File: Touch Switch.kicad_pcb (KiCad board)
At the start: 2 copper layers, 84.8 x 53.2 mm, 55 parts, among them J1 Conn_01x01_Pin, J2 Conn_02x04_Counter_Clockwise, J3 Conn_01x01_Pin, J4 Conn_01x01_Pin, J5 Conn_01x01_Pin, J6 Conn_01x01_Pin, J7 Conn_01x01_Pin, J8 Conn_01x01_Pin, K1 Relay_SPST-NO, K2 Relay_SPST-NO, K3 Relay_SPST-NO, K4 Relay_SPST-NO, Q1 MMBT3904, Q2 MMBT3904, Q3 MMBT3904, Q5 MMBT3904, T1 Transformer_1P_2S, U1 SCJT1117B-3.3-A

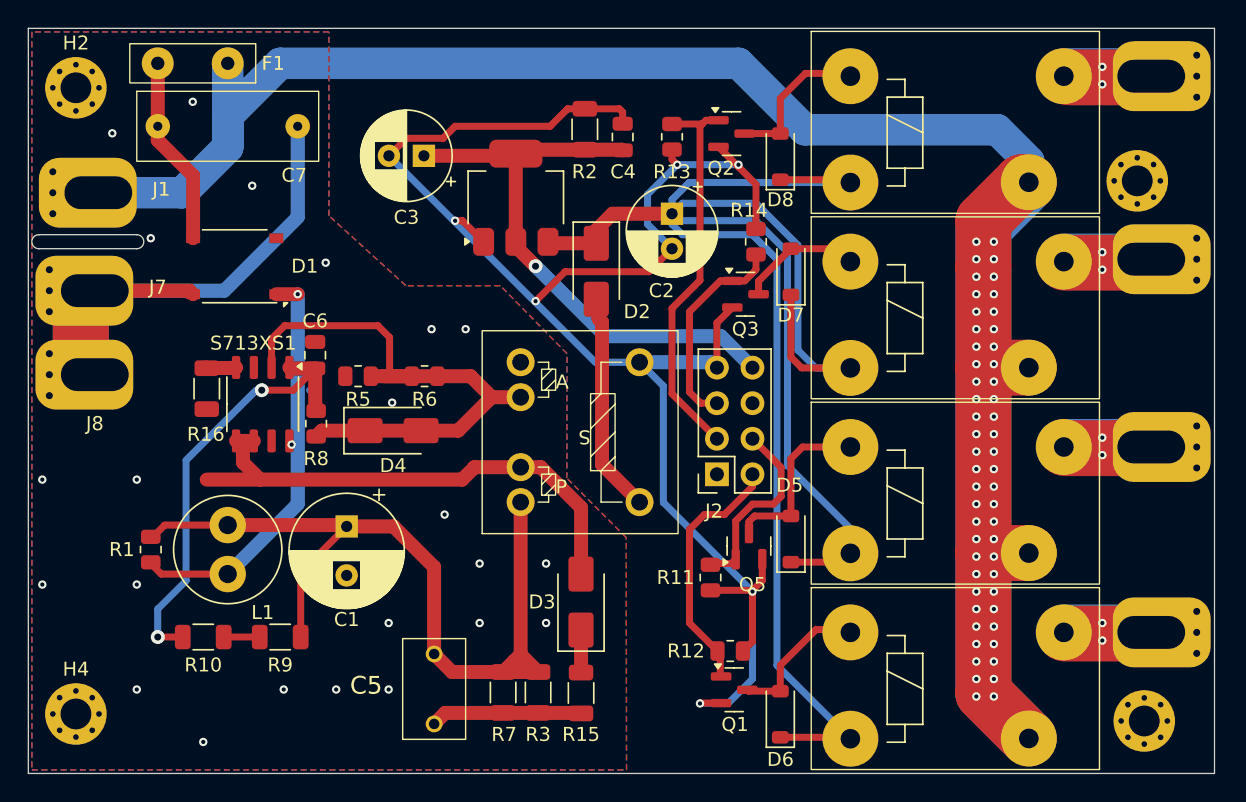
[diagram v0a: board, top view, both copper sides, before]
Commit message: PCB V2
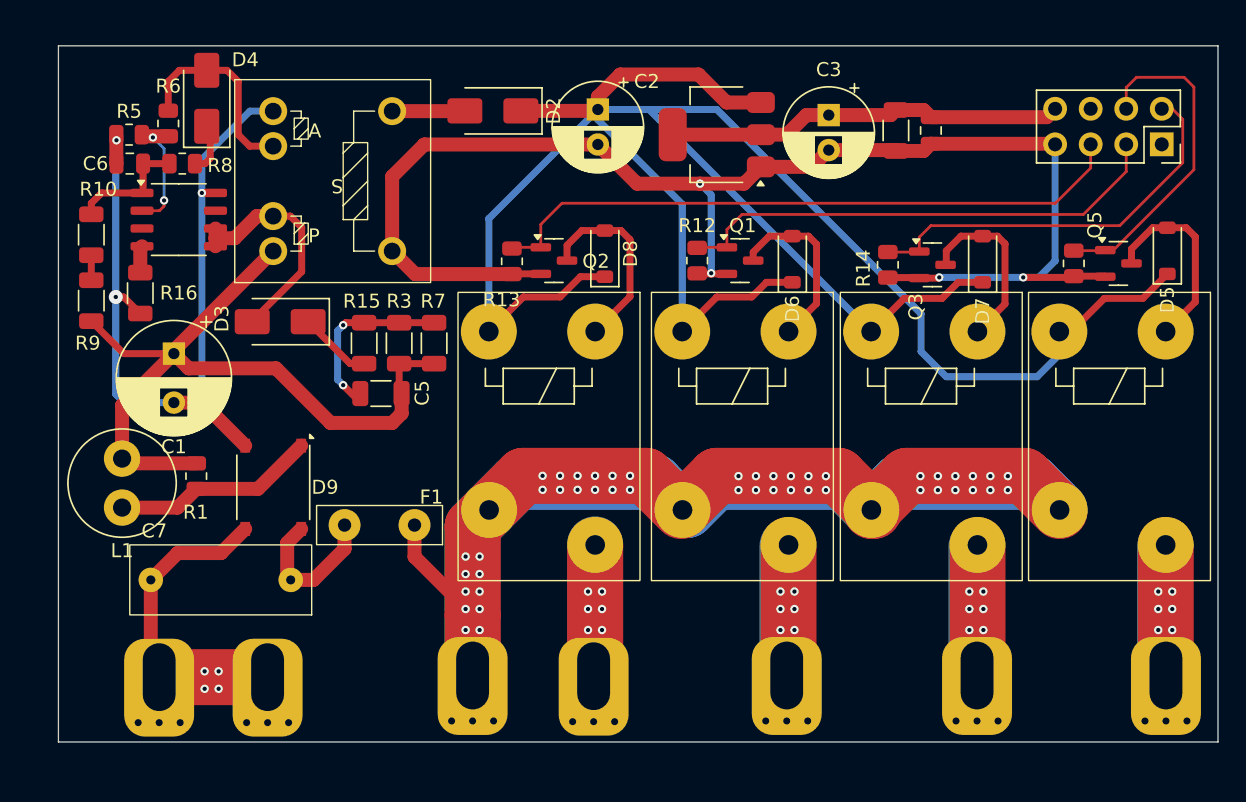
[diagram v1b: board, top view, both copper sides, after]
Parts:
- removed D1: D_Bridge_+-AA, Diode_SMD:Diode_Bridge_Diotec_ABS
- removed H1, H2, H3, H4: MountingHole, MountingHole:MountingHole_2.2mm_M2_Pad_Via
- added D9: DF08M, Diode_SMD:Diode_Bridge_Diotec_ABS, F.Cu at (162.0, 94.8)
- C5: footprint footprint:PFR5101J400J11L4BULK -> Capacitor_SMD:C_1206_3216Metric
- moved J6 58.5 mm to (184.9, 108.3), turned to 0 degrees
- moved J1 43.7 mm to (176.2, 108.2), turned to 0 degrees
- moved J2 39.6 mm to (225.5, 70.3), turned to -90 degrees
- moved K3 36.7 mm to (181.7, 91.2), turned to -90 degrees
- moved F1 35.6 mm to (170.1, 97.5)
- moved R11 34.3 mm to (219.2, 78.8)
- moved D5 33.9 mm to (225.9, 77.9)
- moved Q5 33.2 mm to (222.4, 78.8), turned to 0 degrees
- moved D6 32.5 mm to (199.1, 78.5)
- moved C7 32.4 mm to (158.2, 101.4), turned to 180 degrees
- moved J4 32.3 mm to (212.3, 108.2), turned to 0 degrees
- moved Q1 30.7 mm to (195.4, 78.6)
- moved R10 29.8 mm to (149.0, 76.8), turned to 90 degrees
- moved R15 29.4 mm to (168.5, 84.5), turned to -90 degrees
- moved D3 29.4 mm to (162.5, 83.0), turned to 180 degrees
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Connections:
- F1 pad 1: (no net) -> L
- J1 pad 1: (no net) -> L
- J3 pad 1: (no net) -> R1
- J4 pad 1: (no net) -> R2
- J5 pad 1: (no net) -> R3
- J6 pad 1: (no net) -> R4
- K1 pad 13: (no net) -> L
- K1 pad 14: (no net) -> R1
- K2 pad 13: (no net) -> L
- K2 pad 14: (no net) -> R3
- K3 pad 13: (no net) -> L
- K3 pad 14: (no net) -> R4
- K4 pad 13: (no net) -> L
- K4 pad 14: (no net) -> R2
- Q1 pad 1: CT4 -> CT3
- Q2 pad 1: CT3 -> CT1
- Q3 pad 1: CT1 -> CT4
- R12 pad 1: CT4 -> CT3
- R13 pad 1: CT3 -> CT1
- R14 pad 1: CT1 -> CT4
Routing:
- net GND: track 0.00 -> 59.6 mm, vias 24 -> 3
- net L: track 174.7 -> 125.7 mm, vias 54 -> 46
- net CT1: track 15.1 -> 46.4 mm
- net GND2: track 129.7 -> 103.0 mm, vias 6 -> 4
- net VCC_IC: track 31.8 -> 8.73 mm, vias 2 -> 0
- net N: track 44.3 -> 23.2 mm, vias 0 -> 4
- net Prim: track 37.6 -> 16.8 mm
- net Net-(D9-+): track 29.5 -> 14.6 mm, vias 1 -> 0
- net +5V: track 149.1 -> 162.6 mm
- net +3.3V: track 41.5 -> 28.5 mm, vias 1 -> 0
- net CT4: track 18.3 -> 29.2 mm
- net Sec: track 15.8 -> 4.98 mm
- net CT2: track 13.9 -> 23.8 mm
- net R2: track 14.6 -> 23.8 mm, vias 2 -> 6
- net R3: track 14.7 -> 23.8 mm, vias 2 -> 6
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- removed copper zone on B.Cu, net GND
- removed copper zone on F.Cu, net GND
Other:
- board size 84.8 x 53.2 mm -> 82.9 x 49.8 mm
